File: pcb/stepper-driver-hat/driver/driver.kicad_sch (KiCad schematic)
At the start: 11 parts, among them J1 Conn_01x02, J2 Conn_01x04, J3 Conn_01x04, J4 Conn_01x04, U1 TMC2209_BTT_1.3, U2 TMC2209_BTT_1.3

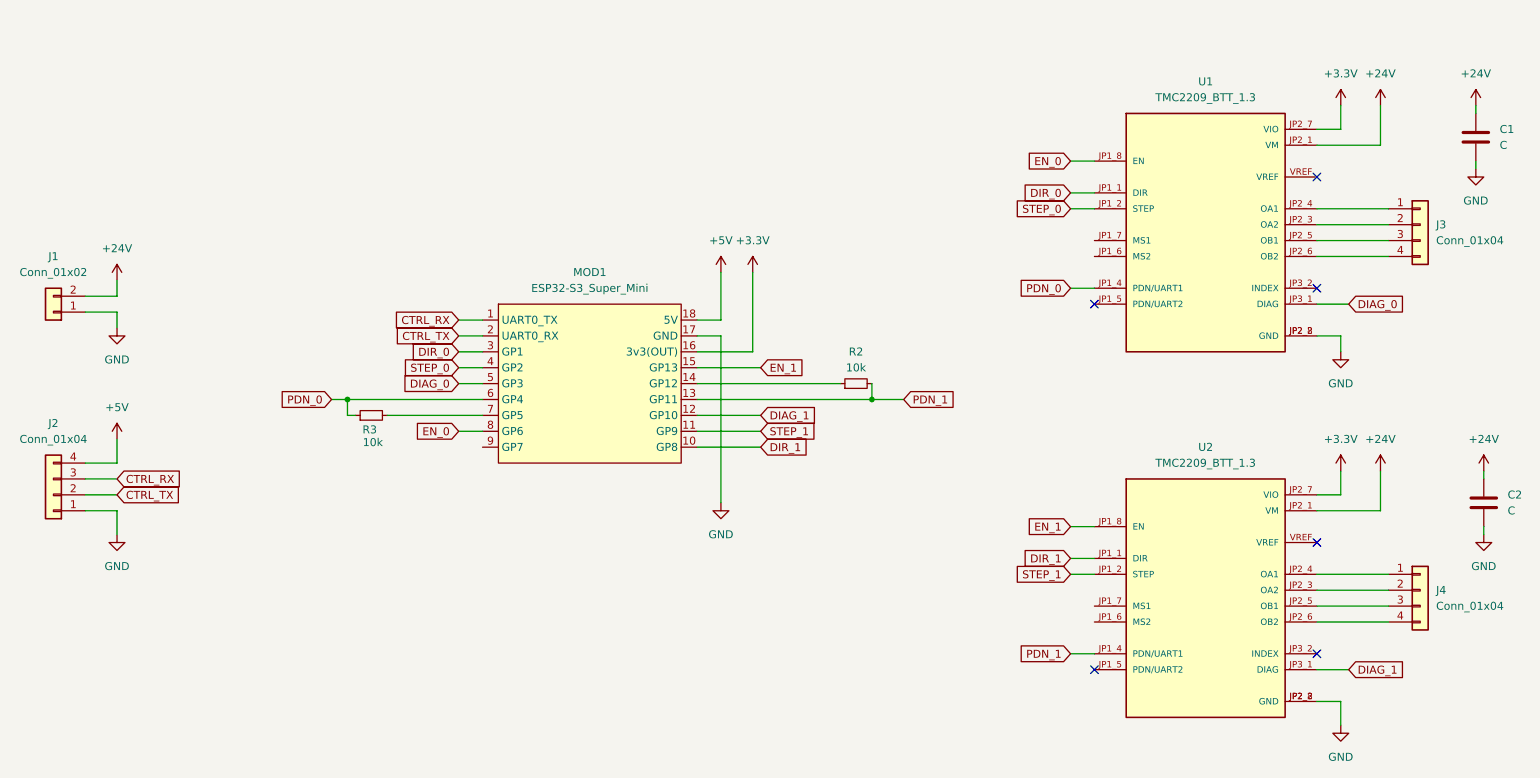
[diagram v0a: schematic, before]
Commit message: firmeware update
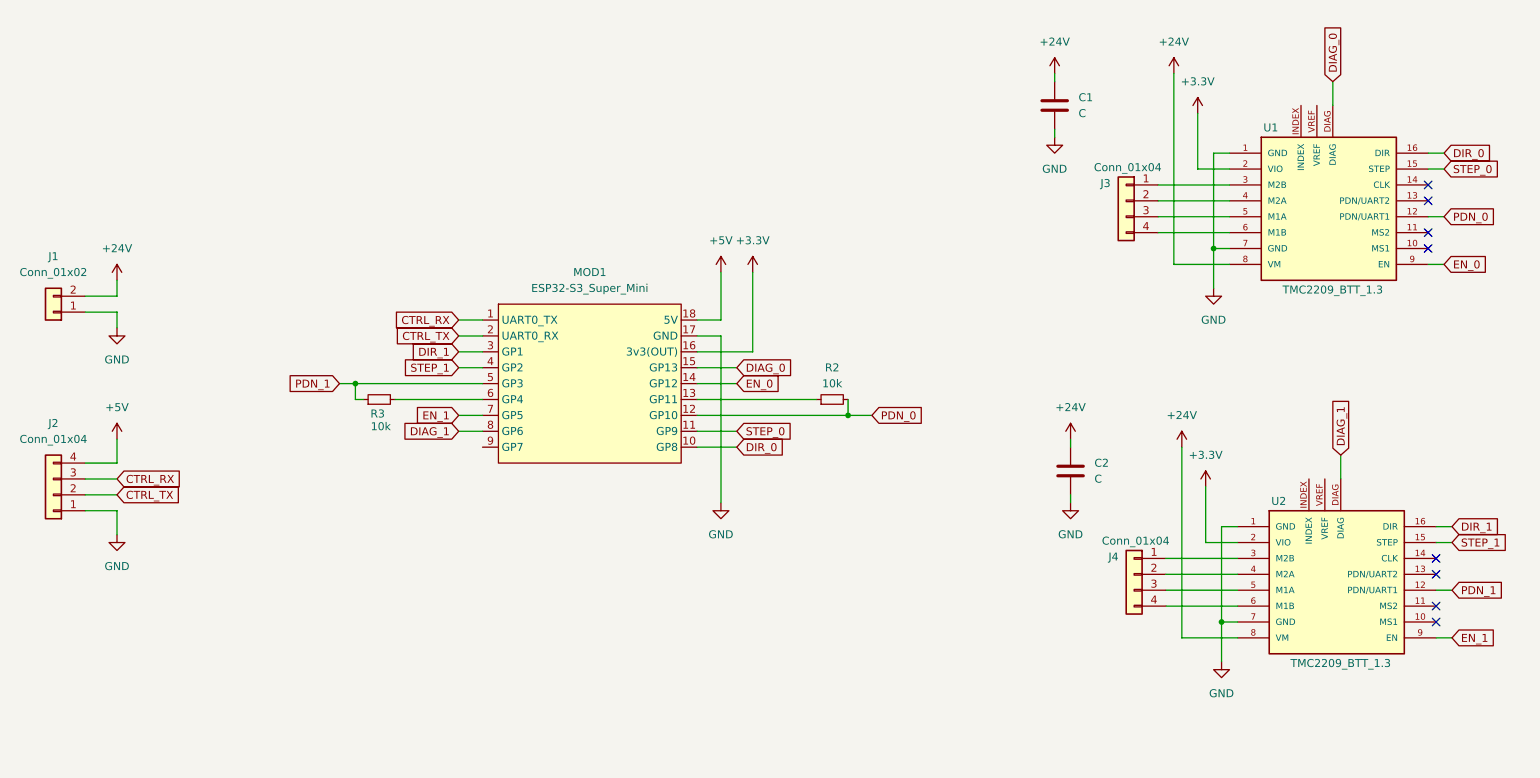
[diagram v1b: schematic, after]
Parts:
- U1, U2: footprint MotorDrivers:MODULE_TMC2208_SILENTSTEPSTICK -> MotorDrivers:MODULE_TMC2208_TMC2209
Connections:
- net +24V: now also U1.8 (VM), U2.8 (VM); no longer U1.JP2_1 (VM), U2.JP2_1 (VM)
- net +3.3V: now also U1.2 (VIO), U2.2 (VIO); no longer U1.JP2_7 (VIO), U2.JP2_7 (VIO)
- net DIAG_0: now also MOD1.15 (GP13), U1.DIAG; no longer MOD1.5 (GP3), U1.JP3_1 (DIAG)
- net DIAG_1: now also MOD1.8 (GP6), U2.DIAG; no longer MOD1.12 (GP10), U2.JP3_1 (DIAG)
- net DIR_0: now also MOD1.10 (GP8), U1.16 (DIR); no longer MOD1.3 (GP1), U1.JP1_1 (DIR)
- net DIR_1: now also MOD1.3 (GP1), U2.16 (DIR); no longer MOD1.10 (GP8), U2.JP1_1 (DIR)
- net EN_0: now also MOD1.14 (GP12), U1.9 (EN); no longer MOD1.8 (GP6), U1.JP1_8 (EN)
- net EN_1: now also MOD1.7 (GP5), U2.9 (EN); no longer MOD1.15 (GP13), U2.JP1_8 (EN)
- net GND: now also U1.1 (GND), U1.7 (GND), U2.1 (GND), U2.7 (GND); no longer U1.JP2_2 (GND), U1.JP2_8 (GND), U2.JP2_2 (GND), U2.JP2_8 (GND)
- net PDN_0: now also MOD1.12 (GP10), R2.2, U1.12 (PDN/UART1); no longer MOD1.6 (GP4), R3.1, U1.JP1_4 (PDN/UART1)
- net PDN_1: now also MOD1.5 (GP3), R3.1, U2.12 (PDN/UART1); no longer MOD1.13 (GP11), R2.2, U2.JP1_4 (PDN/UART1)
- net STEP_0: now also MOD1.11 (GP9), U1.15 (STEP); no longer MOD1.4 (GP2), U1.JP1_2 (STEP)
- net STEP_1: now also MOD1.4 (GP2), U2.15 (STEP); no longer MOD1.11 (GP9), U2.JP1_2 (STEP)
- net at J4.1 (Pin_1): now also U2.3 (M2B); no longer U2.JP2_4 (OA1)
- net at J4.2 (Pin_2): now also U2.4 (M2A); no longer U2.JP2_3 (OA2)
- net at J4.3 (Pin_3): now also U2.5 (M1A); no longer U2.JP2_5 (OB1)
- net at J4.4 (Pin_4): now also U2.6 (M1B); no longer U2.JP2_6 (OB2)
- net at R2.1: now also MOD1.13 (GP11); no longer MOD1.14 (GP12)
- net at R3.2: now also MOD1.6 (GP4); no longer MOD1.7 (GP5)
- net at J3.2 (Pin_2): now also U1.4 (M2A); no longer U1.JP2_3 (OA2)
- net at J3.1 (Pin_1): now also U1.3 (M2B); no longer U1.JP2_4 (OA1)
- net at J3.3 (Pin_3): now also U1.5 (M1A); no longer U1.JP2_5 (OB1)
- net at J3.4 (Pin_4): now also U1.6 (M1B); no longer U1.JP2_6 (OB2)
- no-connect marks 6 -> 8
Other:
- moved on the sheet: C1, C2, J4, R2, R3
